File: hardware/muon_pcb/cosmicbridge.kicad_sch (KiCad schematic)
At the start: 3 parts, among them J1 Conn_Coaxial, J3 Conn_02x02_Top_Bottom

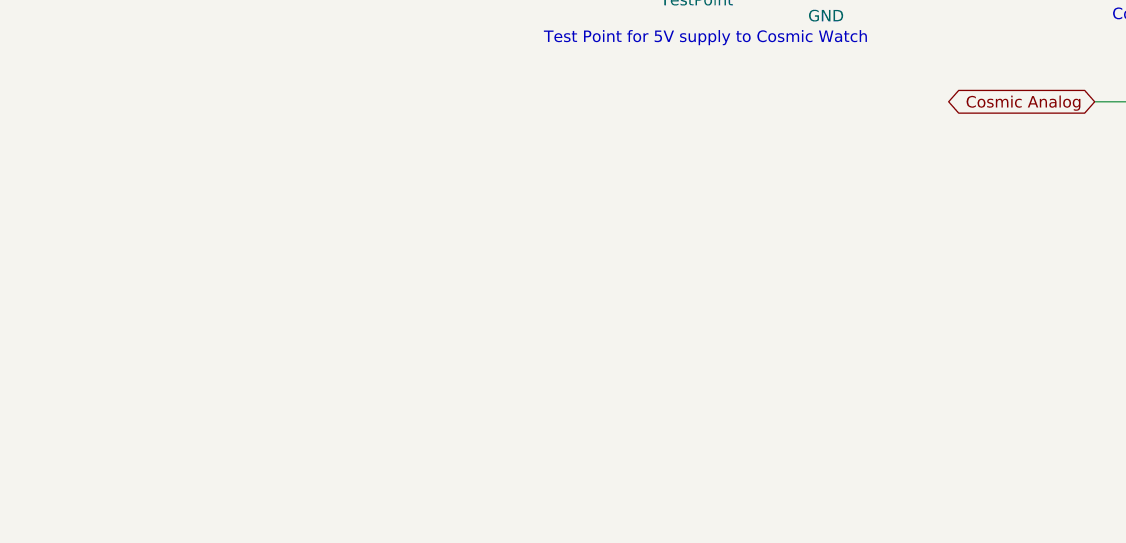
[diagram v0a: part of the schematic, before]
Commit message: updated schematic & cleanup
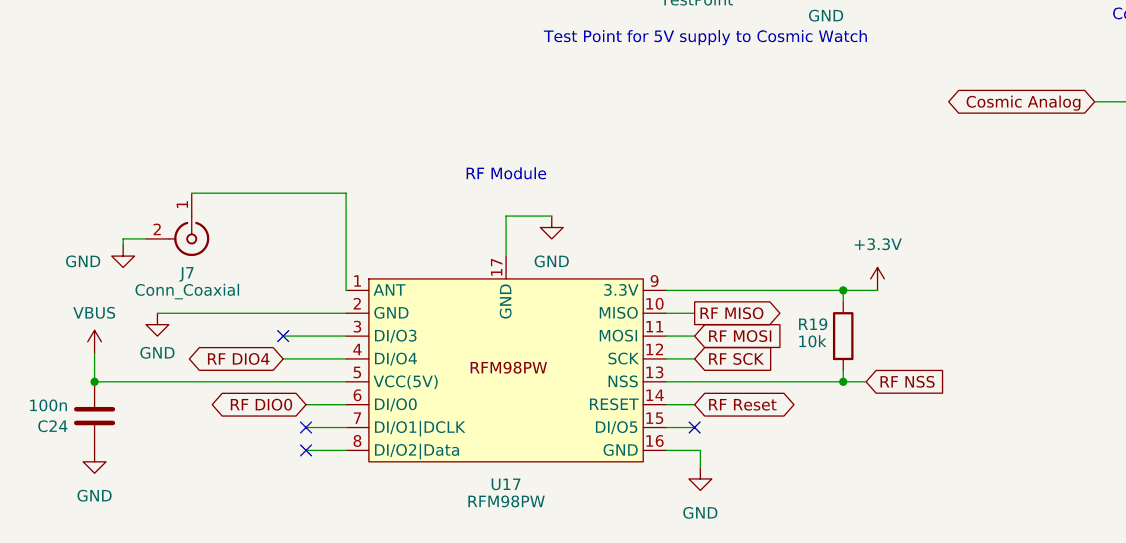
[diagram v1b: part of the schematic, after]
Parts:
- added C24: 100n, Capacitor_SMD:C_0402_1005Metric, symbol Device:C
- added J7: Conn_Coaxial, Connector_Coaxial:SMA_Amphenol_901-144_Vertical, symbol Connector:Conn_Coaxial
- added R19: 10k, Resistor_SMD:R_0402_1005Metric, symbol Device:R
- added U17: RFM98PW, 1my_footprints:RFM98PW, symbol 1my_symbol:RF_Module
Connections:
- net GND: now also C24.1, J7.2 (Ext), U17.16 (GND), U17.17 (GND), U17.2 (GND)
- net VBUS: now also C24.2, U17.5 (VCC(5V))
- new net: J7.1 (In), U17.1 (ANT)
- new net +3.3V: R19.1, U17.9 (3.3V)
- new net RF DIO0: U17.6 (DI/O0)
- new net RF DIO4: U17.4 (DI/O4)
- new net RF MISO: U17.10 (MISO)
- new net RF MOSI: U17.11 (MOSI)
- new net RF NSS: R19.2, U17.13 (NSS)
- new net RF Reset: U17.14 (RESET)
- new net RF SCK: U17.12 (SCK)
- no-connect marks 0 -> 4
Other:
- note added: "RF Module"

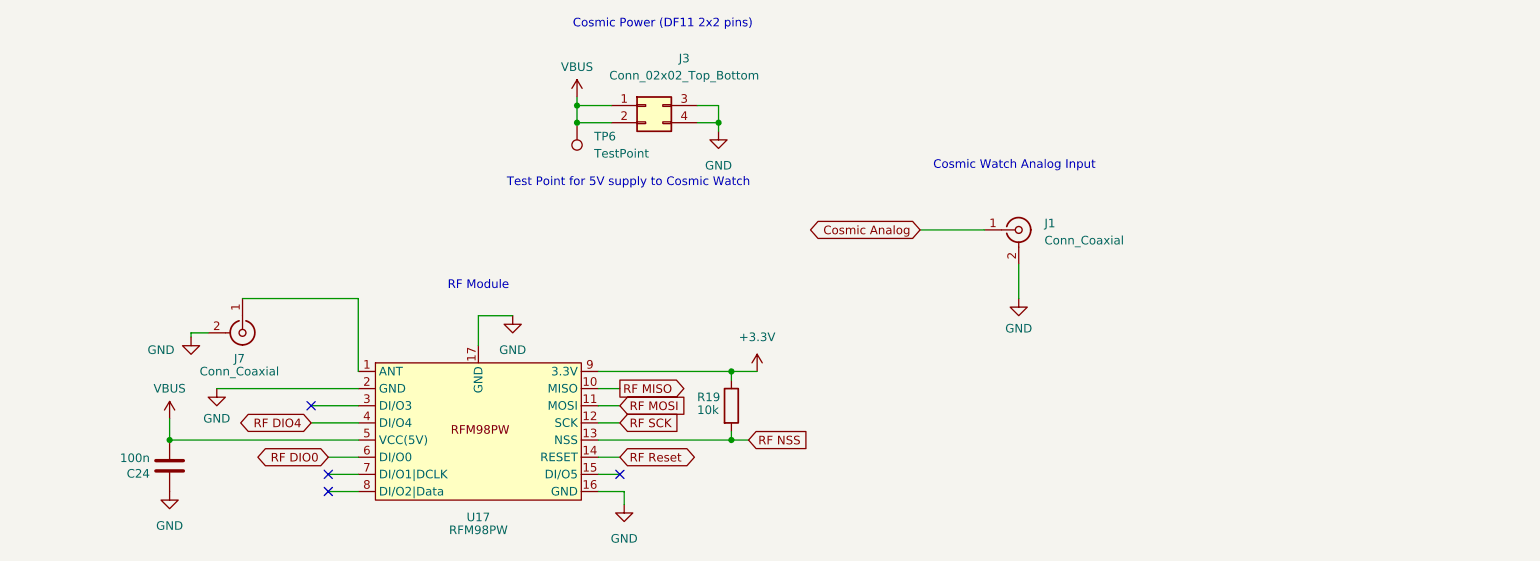
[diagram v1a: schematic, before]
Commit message: uploaded cleaner schematic
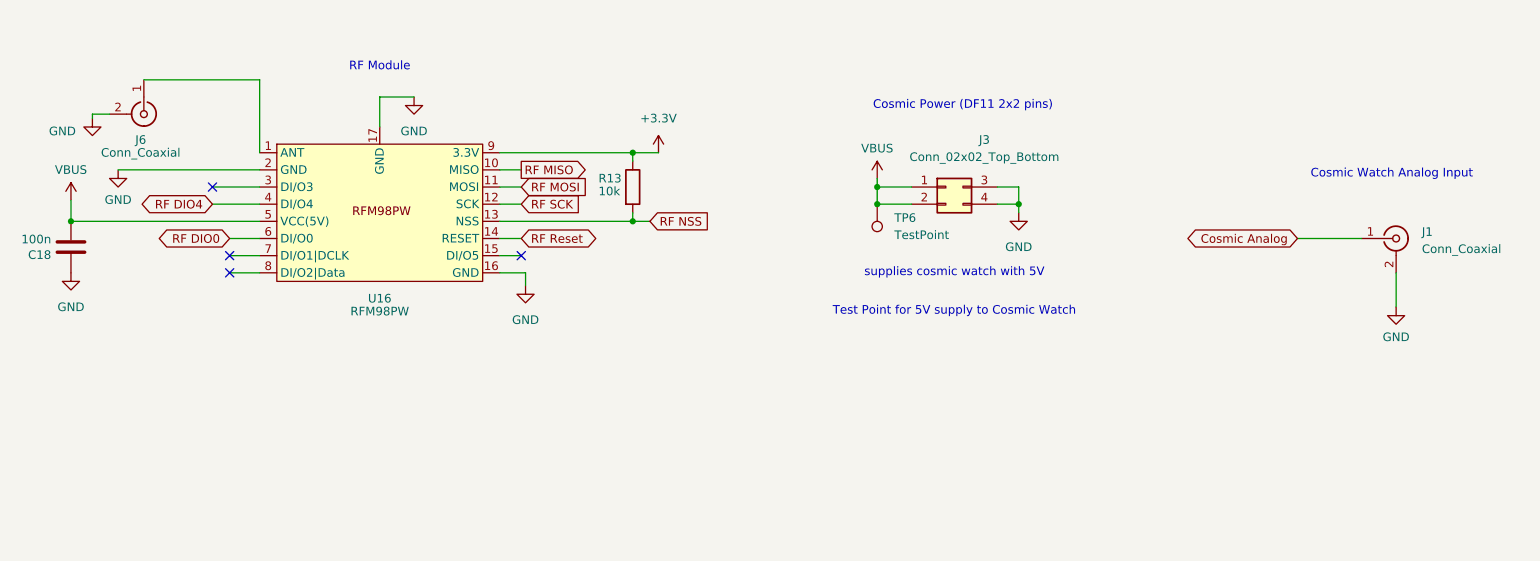
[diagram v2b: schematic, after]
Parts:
- renumbered C24 to C18, J7 to J6, R19 to R13, U17 to U16
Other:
- note added: "supplies cosmic watch with 5V"
- moved on the sheet: C18, J1, J3, J6, R13, TP6, U16
